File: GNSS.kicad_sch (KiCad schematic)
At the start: 0 parts

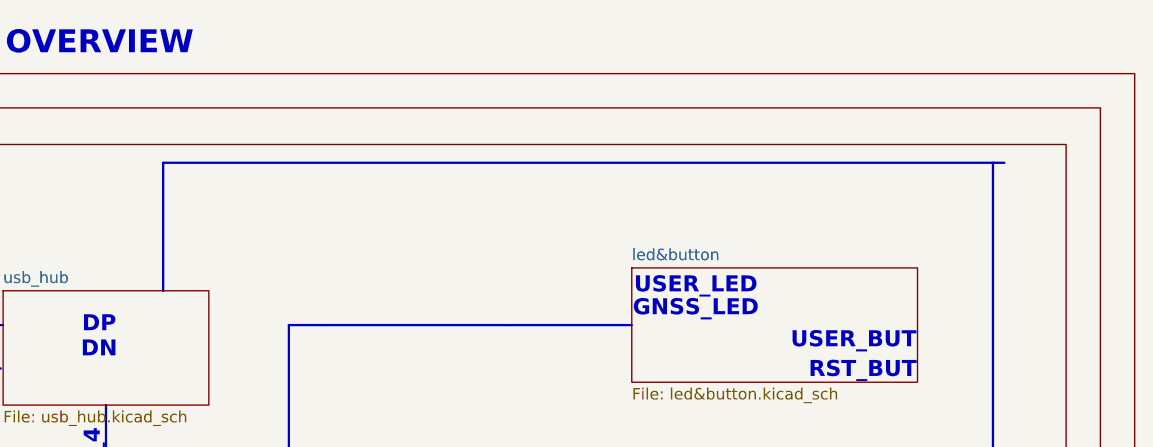
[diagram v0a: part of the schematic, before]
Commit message: new
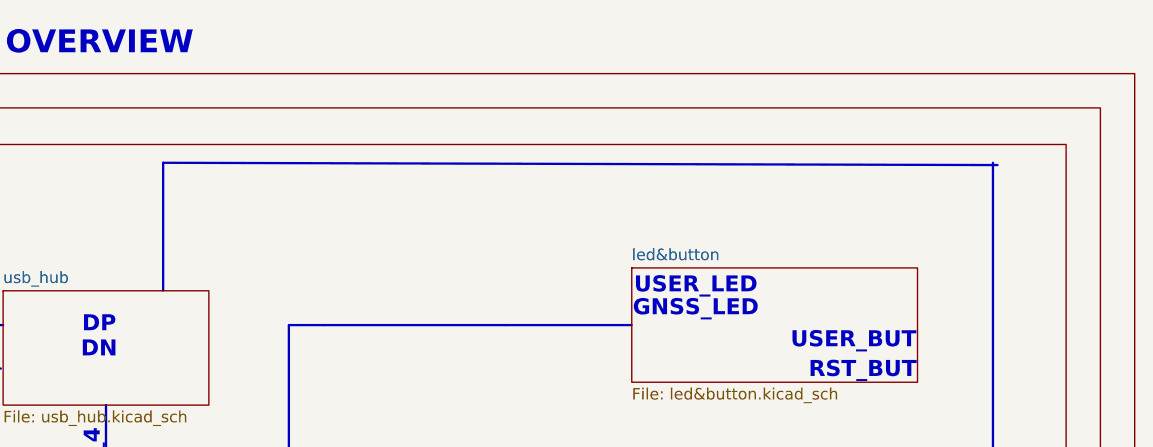
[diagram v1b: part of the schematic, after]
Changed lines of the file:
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@@
 	(polyline
 		(pts
-			(xy 167.64 31.496) (xy 261.112 31.496)
+			(xy 167.64 31.496) (xy 260.35 31.75)
 		)
 		(stroke
